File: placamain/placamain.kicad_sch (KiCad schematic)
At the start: 66 parts, among them J1 Conn_01x10_Pin, J2 Conn_01x10_Pin, J3 Conn_01x12_Pin, J8 Conn_01x10_Pin, Q1 PN3643, Q2 BC559, U1 LM393, U10 LF356, U11 DG211CJ, U12 LF356, U2 LF356, U3 LF356, U4 LF356, U5 AD548JN, U6 LF356, U7 LF356, U8 LM393, U9 LM393

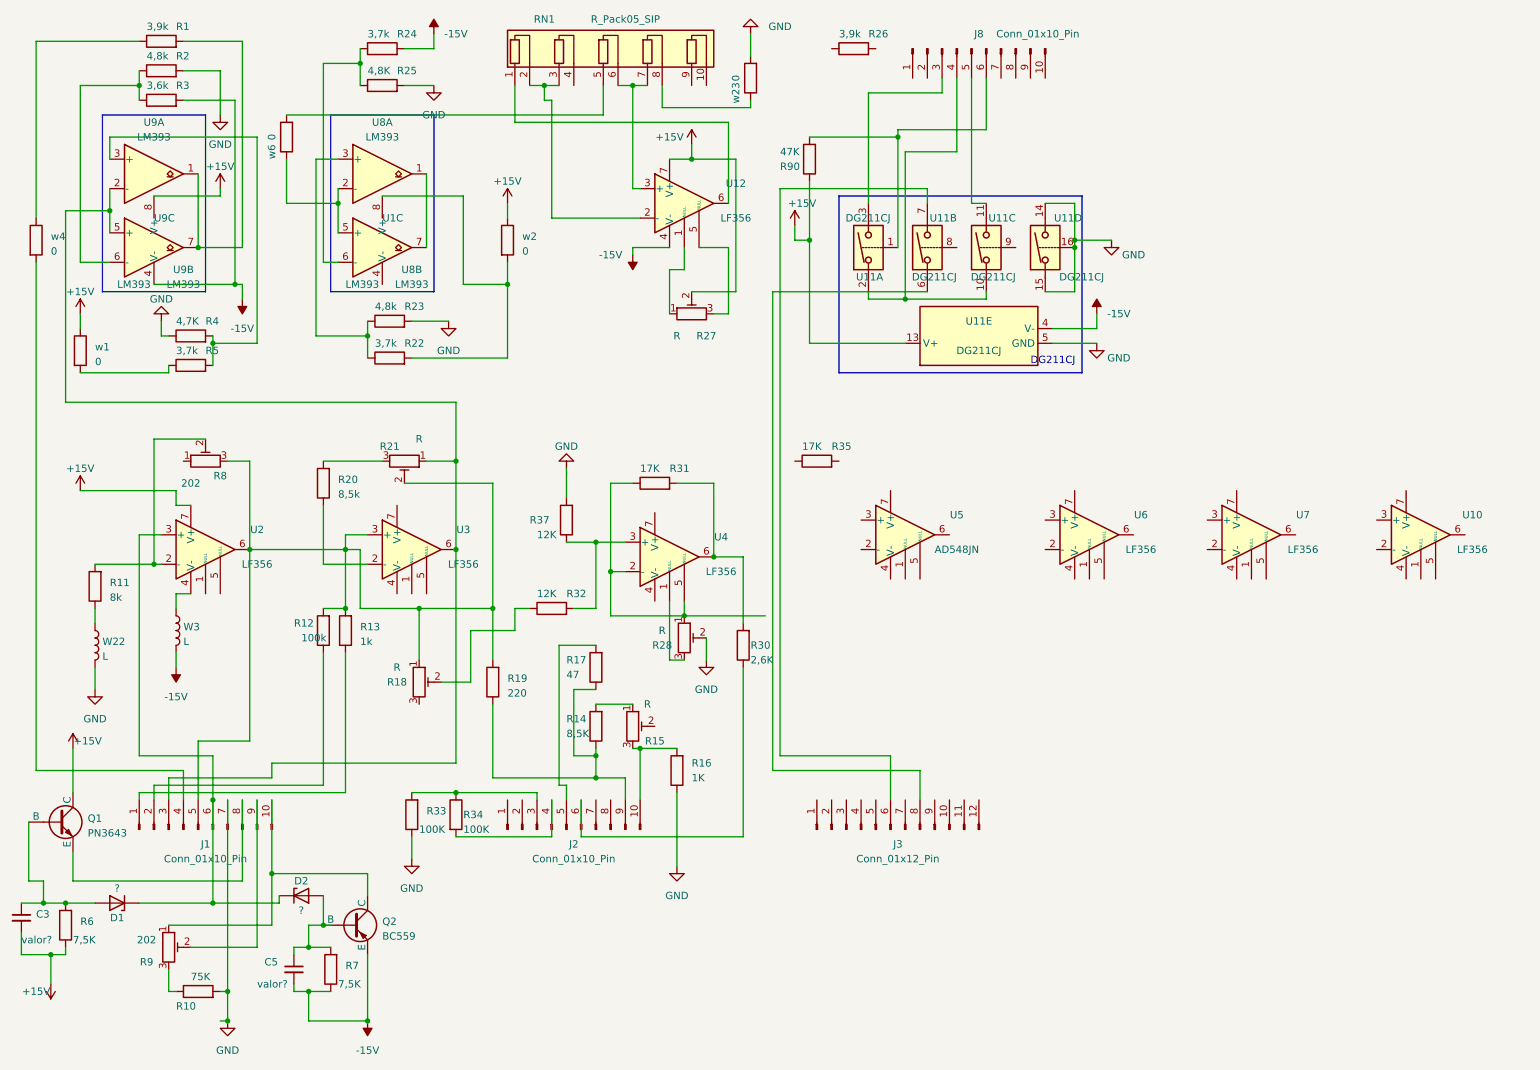
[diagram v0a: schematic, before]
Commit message: pureba de equipo funcionando
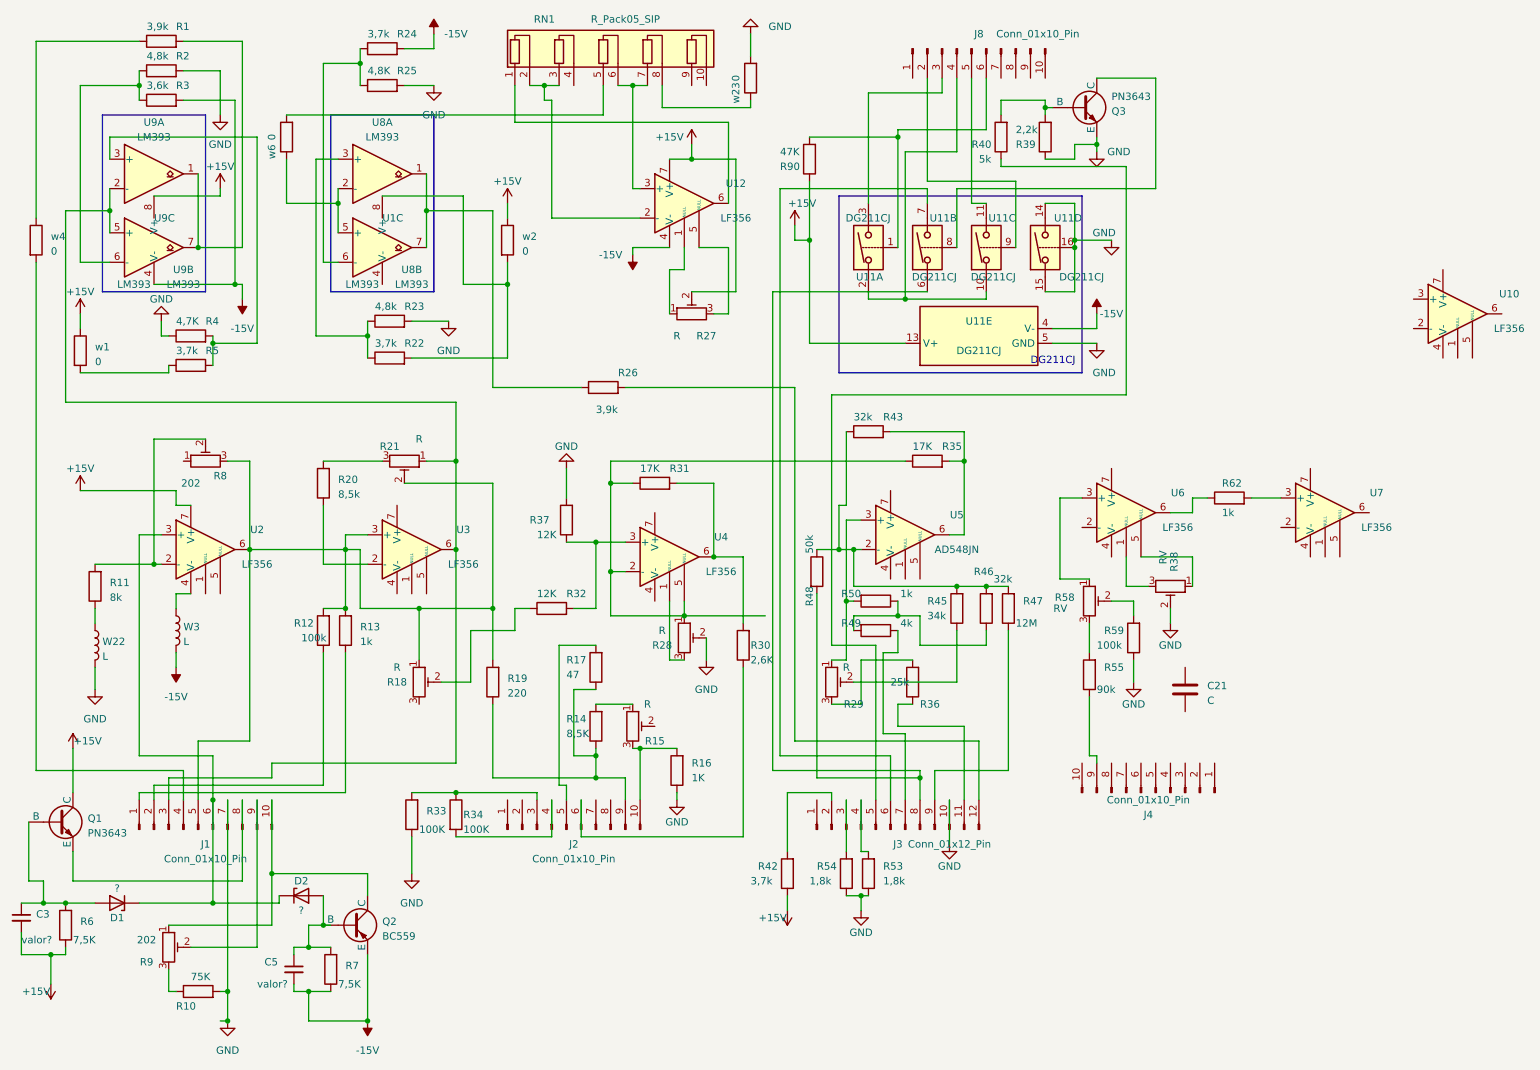
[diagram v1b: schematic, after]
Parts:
- added C21: C, symbol Device:C
- added J4: Conn_01x10_Pin, symbol Connector:Conn_01x10_Pin
- added Q3: PN3643, symbol Simulation_SPICE:NPN
- added R29: R, symbol Device:R_Potentiometer_Trim
- added R36: 25k, symbol Device:R
- added R38, R58: RV, symbol Device:R_Potentiometer_Trim
- added R39: 2,2k, symbol Device:R
- added R40: 5k, symbol Device:R
- added R42: 3,7k, symbol Device:R
- added R43, R46: 32k, symbol Device:R
- added R45: 34k, symbol Device:R
- added R47: 12M, symbol Device:R
- added R48: 50k, symbol Device:R
- added R49: 4k, symbol Device:R
- added R50, R62: 1k, symbol Device:R
- added R53, R54: 1,8k, symbol Device:R
- added R55: 90k, symbol Device:R
- added R59: 100k, symbol Device:R
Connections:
- net +15V: now also R42.1
- net GND: now also J3.10 (Pin_10), Q3.3 (E), R38.2, R39.1, R53.1, R54.1, R59.1
- net at R28.1, R31.1, U4.2 (-)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: now also R35.1
- net at R26.1: now also U8.1, U8.7
- net at R26.2: now also J3.12 (Pin_12)
- net at J3.11 (Pin_11): now also R36.1
- net at J3.2 (Pin_2): now also R42.2
- net at J3.3 (Pin_3): now also R54.2
- net at J3.4 (Pin_4): now also R53.2
- net at J3.5 (Pin_5): now also R40.1
- net at J3.7 (Pin_7): now also R49.1
- net at J3.8 (Pin_8), U11.6: now also R48.2
- net at J3.9 (Pin_9): now also R47.1
- net at U11.8: now also Q3.1 (C)
- net at U5.2 (-): now also R43.1, R45.2, R46.2, R47.2, R48.1
- net at U5.3 (+): now also R29.1, R50.2
- net at U5.6: now also R35.2, R43.2
- net at U7.3 (+): now also R62.2
- net at U11.9: now also J8.2 (Pin_2)
- net at U6.1 (NULL): now also R38.3
- net at U6.3 (+): now also R58.1
- net at U6.5 (NULL): now also R38.1
- net at U6.6: now also R62.1
- new net: R29.2, R45.1
- new net: R29.3, R36.2
- new net: R58.2, R59.2
- new net: R55.2, R58.3
- new net: R46.1, R49.2, R50.1
- new net: J4.9 (Pin_9), R55.1
- new net: Q3.2 (B), R39.2, R40.2
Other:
- moved on the sheet: R26, R35, U10, U6, U7
